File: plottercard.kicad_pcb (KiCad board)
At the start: 4 copper layers, 85.7 x 76.2 mm, 70 parts, among them J10 SLTpad, J11 SLTpad, J12 SLTpad, J13 SLTpad, J2 SLTpad, J3 SLTpad, J4 SLTpad, J5 SLTpad, J6 SLTpad, J7 SLTpad, J8 SLTpad, J9 SLTpad, U20 74LS05, U21 LD1117S50TR_SOT223, U6 74LS07, X1 Conn_01x09_Socket, X2 Conn_01x09_Socket, X3 Conn_01x09_Socket, X4 Conn_01x09_Socket

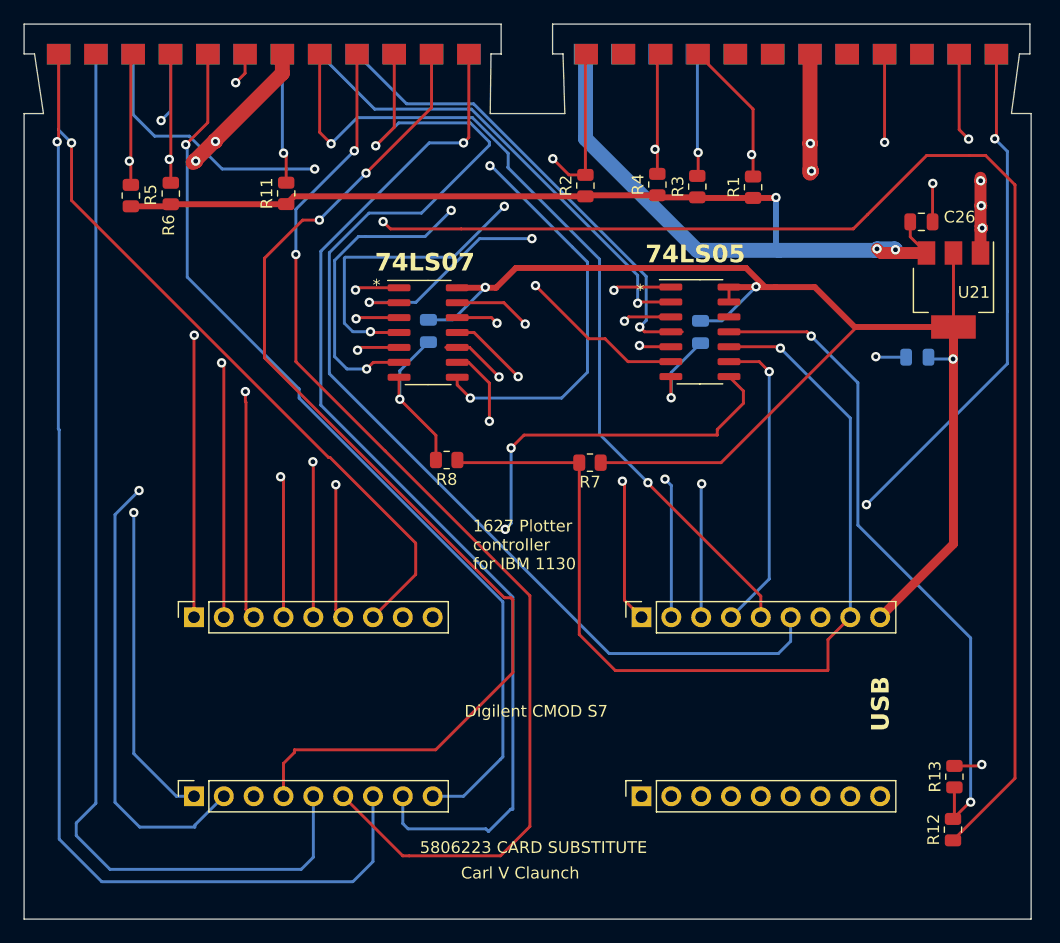
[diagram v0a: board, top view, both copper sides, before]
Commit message: Up to date KiCad design files
matching the gerbers and drill files
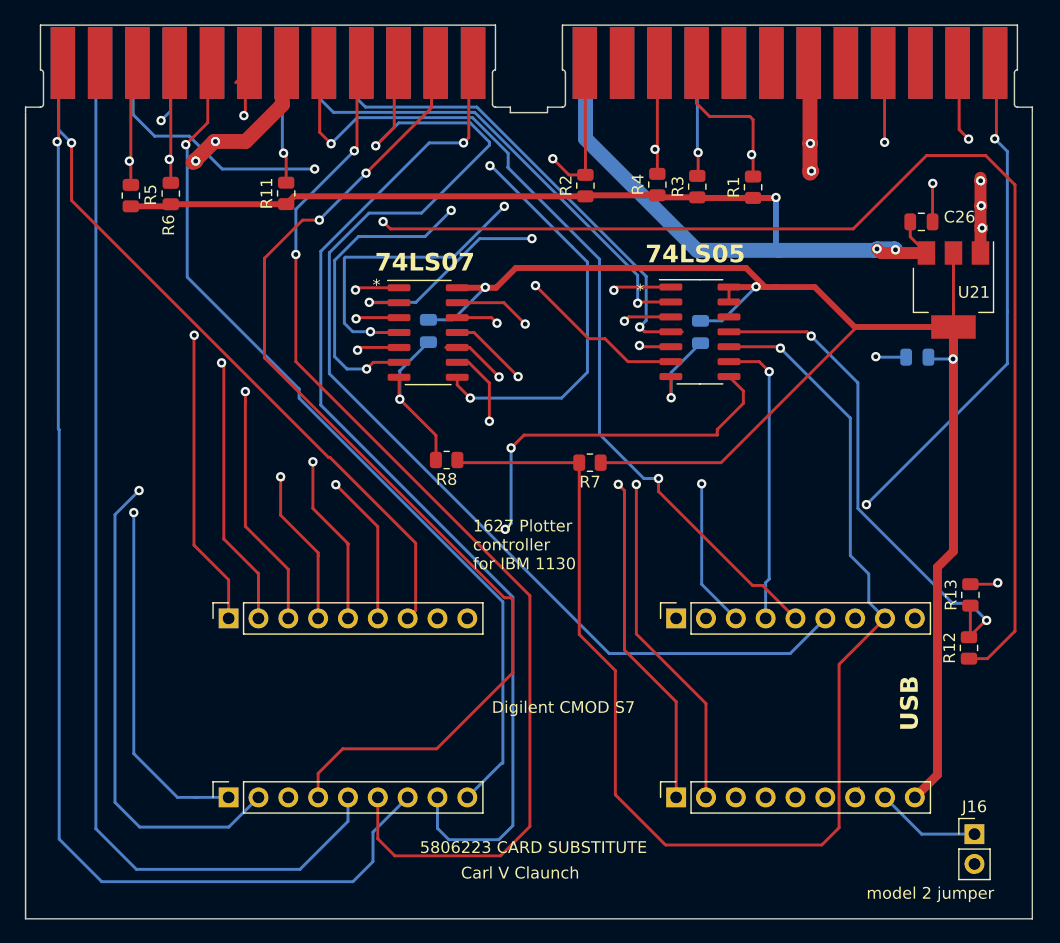
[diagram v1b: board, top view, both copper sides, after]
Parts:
- removed B10, B11, B12, B13, B2, B3, B4, B5, B6, B7, B8, B9, D10, D11, D12, D13, D2, D3, D4, D5, D6, D7, D8, D9, G10, G11, G12, G13, G2, G3, G4, G5, G6, G7, G8, G9, J10, J11, J12, J13, J2, J3, J4, J5, J6, J7, J8, J9: SLTpad, Library.carl:SLTpad
- added J14: EdgeConnectorSingle, IBM:PlugConnector, F.Cu at (82.5, 42.9)
- added J15: EdgeConnectorSingle2, IBM:PlugConnector2, F.Cu at (126.9, 42.9)
- added J16: Conn_01x02_Pin, Connector_PinHeader_2.54mm:PinHeader_1x02_P2.54mm_Vertical, F.Cu at (142.7, 104.8)
- moved X3 15.6 mm to (117.2, 101.7)
- moved R12 15.5 mm to (142.2, 89.0)
- moved R13 15.5 mm to (142.3, 84.5)
- moved X4 15.4 mm to (117.2, 86.5)
- moved X1 2.95 mm to (79.2, 101.7)
- moved X2 2.95 mm to (79.2, 86.5)
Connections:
- R7 pad 2: Net-(X3-Pin_8) -> Net-(X4-Pin_8)
- R8 pad 1: Net-(X3-Pin_8) -> Net-(X4-Pin_8)
- U20 pad 10: Net-(X3-Pin_8) -> Net-(X4-Pin_8)
- U20 pad 5: Net-(X3-Pin_3) -> Net-(X4-Pin_3)
- U20 pad 9: Net-(X3-Pin_4) -> Net-(X4-Pin_4)
- X3 pad 3: Net-(X3-Pin_3) -> unconnected-(X3-Pin_3-Pad3)
- X3 pad 4: Net-(X3-Pin_4) -> unconnected-(X3-Pin_4-Pad4)
- X3 pad 5: Net-(D9-Pin_1) -> unconnected-(X3-Pin_5-Pad5)
- X3 pad 6: Net-(D11-Pin_1) -> unconnected-(X3-Pin_6-Pad6)
- X3 pad 8: Net-(X3-Pin_8) -> Net-(J16-Pin_1)
- X4 pad 3: unconnected-(X4-Pin_3-Pad3) -> Net-(X4-Pin_3)
- X4 pad 4: unconnected-(X4-Pin_4-Pad4) -> Net-(X4-Pin_4)
- X4 pad 5: unconnected-(X4-Pin_5-Pad5) -> Net-(X4-Pin_5)
- X4 pad 6: unconnected-(X4-Pin_6-Pad6) -> Net-(X4-Pin_6)
- X4 pad 8: unconnected-(X4-Pin_8-Pad8) -> Net-(X4-Pin_8)
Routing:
- net Net-(X4-Pin_6): track 0.00 -> 120.5 mm, vias 0 -> 2
- net Net-(D11-Pin_1): track 116.1 -> 0.00 mm, vias 2 -> 0
- net Net-(X4-Pin_8): track 0.00 -> 112.7 mm, vias 0 -> 1
- net Net-(X3-Pin_8): track 83.3 -> 0.00 mm, vias 1 -> 0
- net Net-(X4-Pin_5): track 0.00 -> 76.3 mm, vias 0 -> 2
- net Net-(D9-Pin_1): track 73.8 -> 0.00 mm, vias 2 -> 0
- net Net-(X4-Pin_3): track 0.00 -> 29.4 mm, vias 0 -> 2
- net Net-(X3-Pin_3): track 28.1 -> 0.00 mm, vias 2 -> 0
- net Net-(X3-Pin_4): track 26.0 -> 0.00 mm, vias 1 -> 0
- net Net-(X4-Pin_4): track 0.00 -> 24.9 mm, vias 0 -> 1
- net Net-(X3-Pin_1): track 33.8 -> 50.3 mm
- net Net-(X3-Pin_2): track 31.9 -> 48.5 mm
- net Net-(J14-PadB08): track 137.6 -> 122.5 mm
- net Net-(R12-Pad2): track 57.3 -> 43.0 mm
- net Net-(U20G-VCC): track 127.4 -> 141.5 mm
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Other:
- board size 85.7 x 76.2 mm -> 85.7 x 68.7 mm
- board text added: "model 2 jumper"
